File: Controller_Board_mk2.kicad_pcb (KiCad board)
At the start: 2 copper layers, 130.2 x 80.6 mm, 48 parts, among them J1 Barrel_Jack_MountingPin, J2 Barrel_Jack_MountingPin, J3 Barrel_Jack_MountingPin, J4 Barrel_Jack_MountingPin, J5 Barrel_Jack_MountingPin, K1 SANYOU_SRD_Form_C, K2 SANYOU_SRD_Form_C, K3 SANYOU_SRD_Form_C, K4 SANYOU_SRD_Form_C, Q1 BC817, Q2 BC817, Q3 BC817, Q4 BC817, U1 AP63205WU

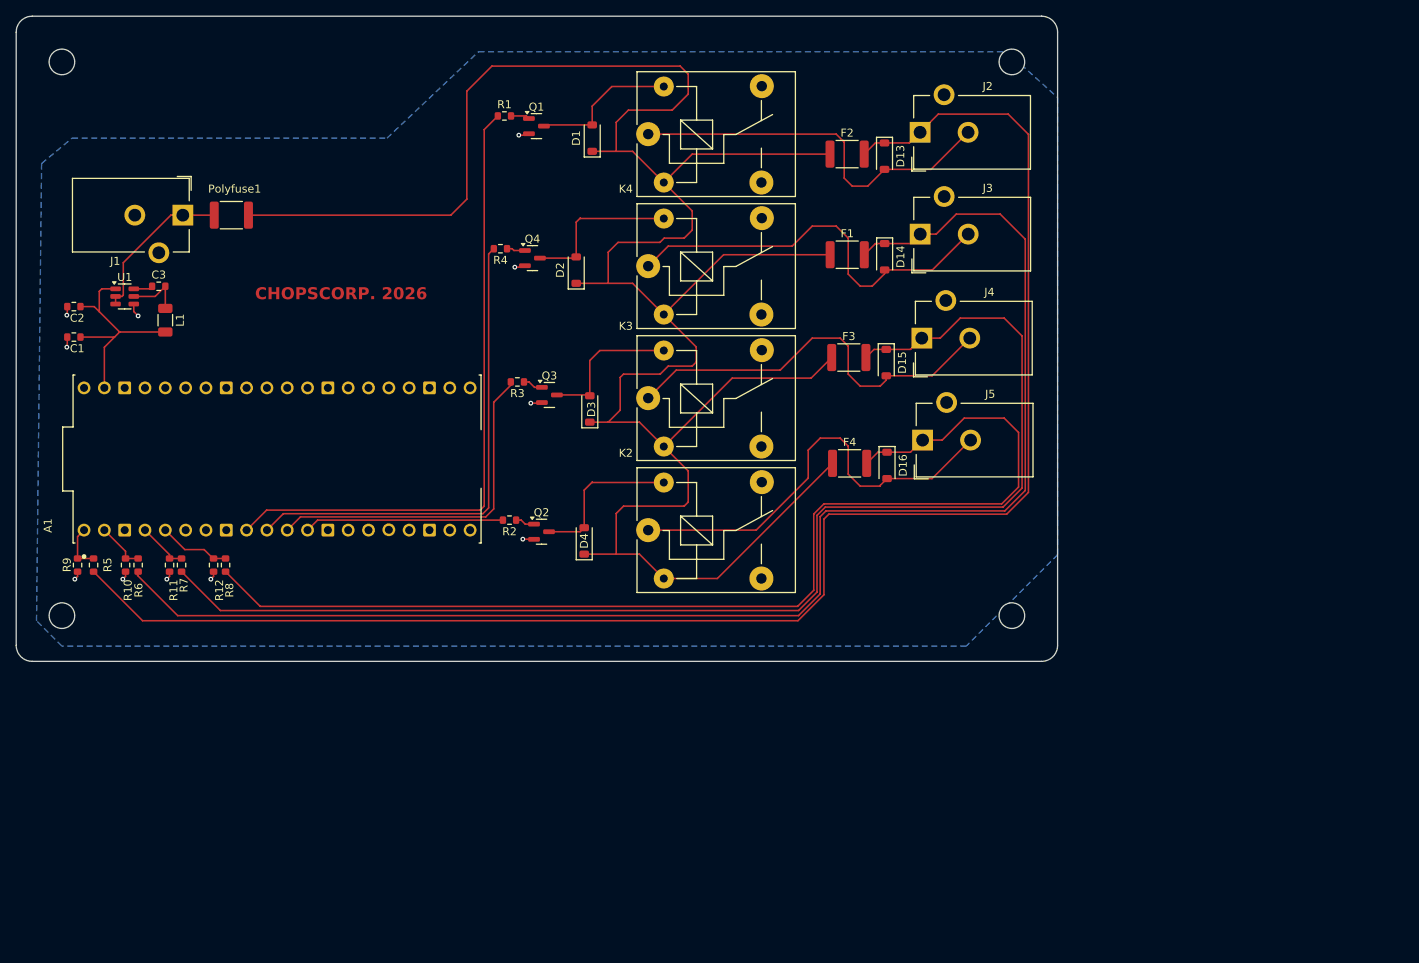
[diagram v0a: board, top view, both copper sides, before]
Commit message: minor fixes
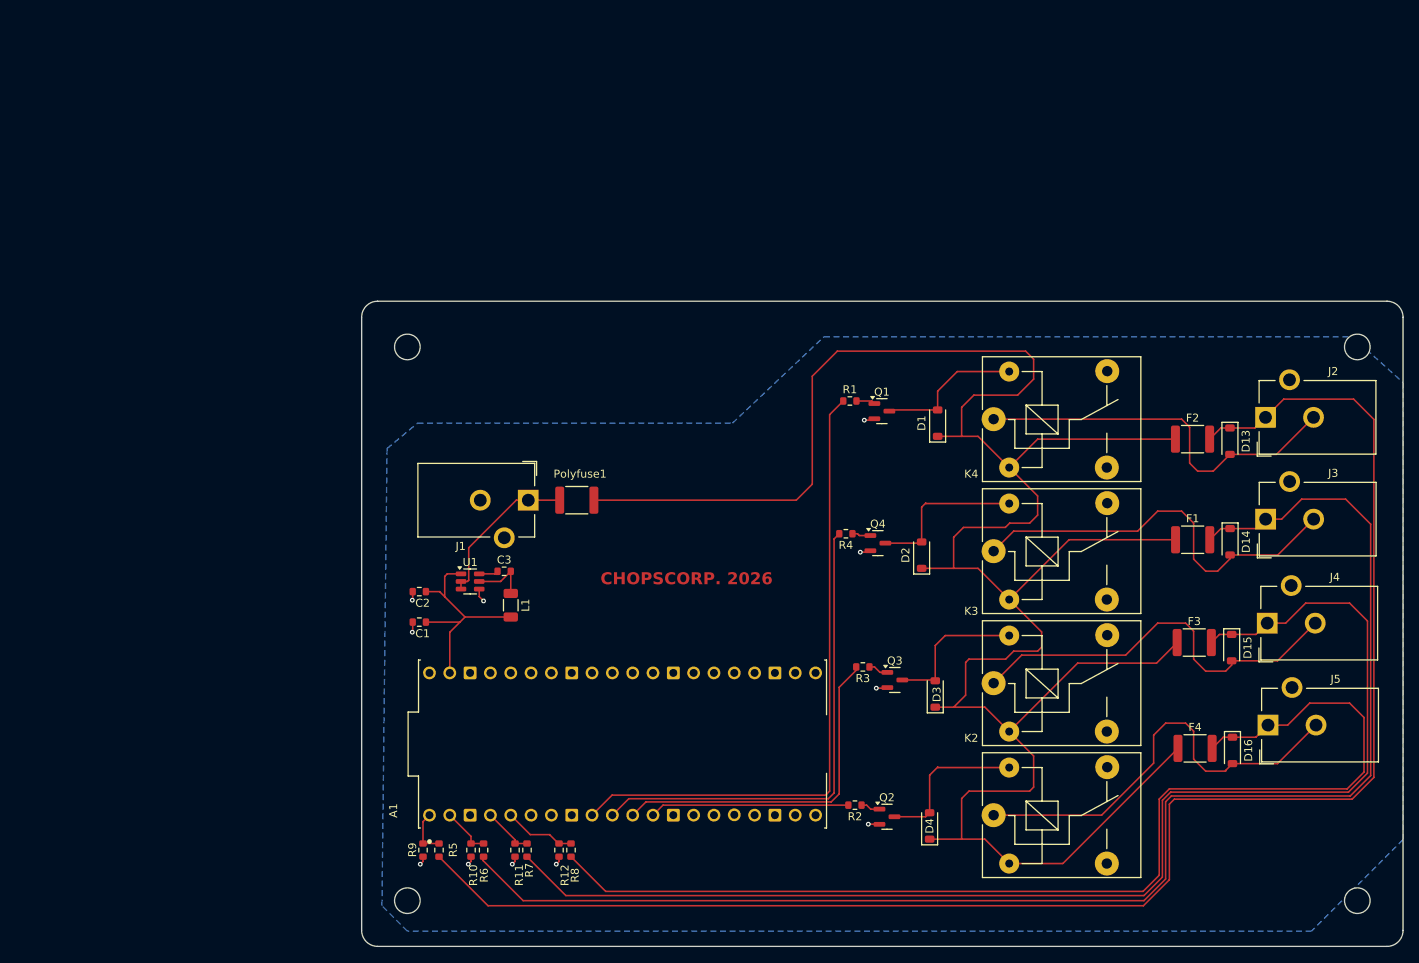
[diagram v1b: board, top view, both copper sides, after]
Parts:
- moved A1 56.0 mm to (75.8, 91.0)
- moved D14 56.0 mm to (151.7, 65.7)
- moved D2 56.0 mm to (113.2, 67.4)
- moved K1 56.0 mm to (122.2, 99.9)
- moved K2 56.0 mm to (122.2, 83.4)
- moved K3 56.0 mm to (122.2, 66.9)
- moved C1 56.0 mm to (50.4, 75.7)
- moved C2 56.0 mm to (50.4, 71.9)
- moved D1 56.0 mm to (115.2, 50.9)
- moved D15 56.0 mm to (151.9, 78.9)
- moved D4 56.0 mm to (114.2, 101.2)
- moved F1 56.0 mm to (147.1, 65.4)
- moved J1 56.0 mm to (64.0, 60.5)
- moved J3 56.0 mm to (156.2, 62.9)
- moved K4 56.0 mm to (122.2, 50.4)
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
